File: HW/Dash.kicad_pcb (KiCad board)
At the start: 4 copper layers, 81 x 56 mm, 104 parts, among them J1 Conn_02x05_Top_Bottom, J2 souriau18pin, Q1 Q_NMOS_GSD, Q10 Q_NMOS_GSD, Q11 Q_NMOS_GSD, Q12 BC857BDW1, Q13 Q_PMOS_GSD, Q14 Q_NMOS_GSD, Q15 Q_NMOS_GSD, Q2 Q_NMOS_GSD, Q3 Q_NMOS_GSD, Q4 Q_NMOS_GSD, Q5 Q_NMOS_GSD, Q6 Q_NMOS_GSD, Q7 Q_NMOS_GSD, Q8 Q_NMOS_GSD, Q9 Q_NMOS_GSD, SW1 SW_Push_Dual, U1 STM32F303VCTx, U2 SN65HVD234, U3 LM1117-3.3, U4 24AA02-OT, U5 LMZ14202TZE-ADJ_NOPB

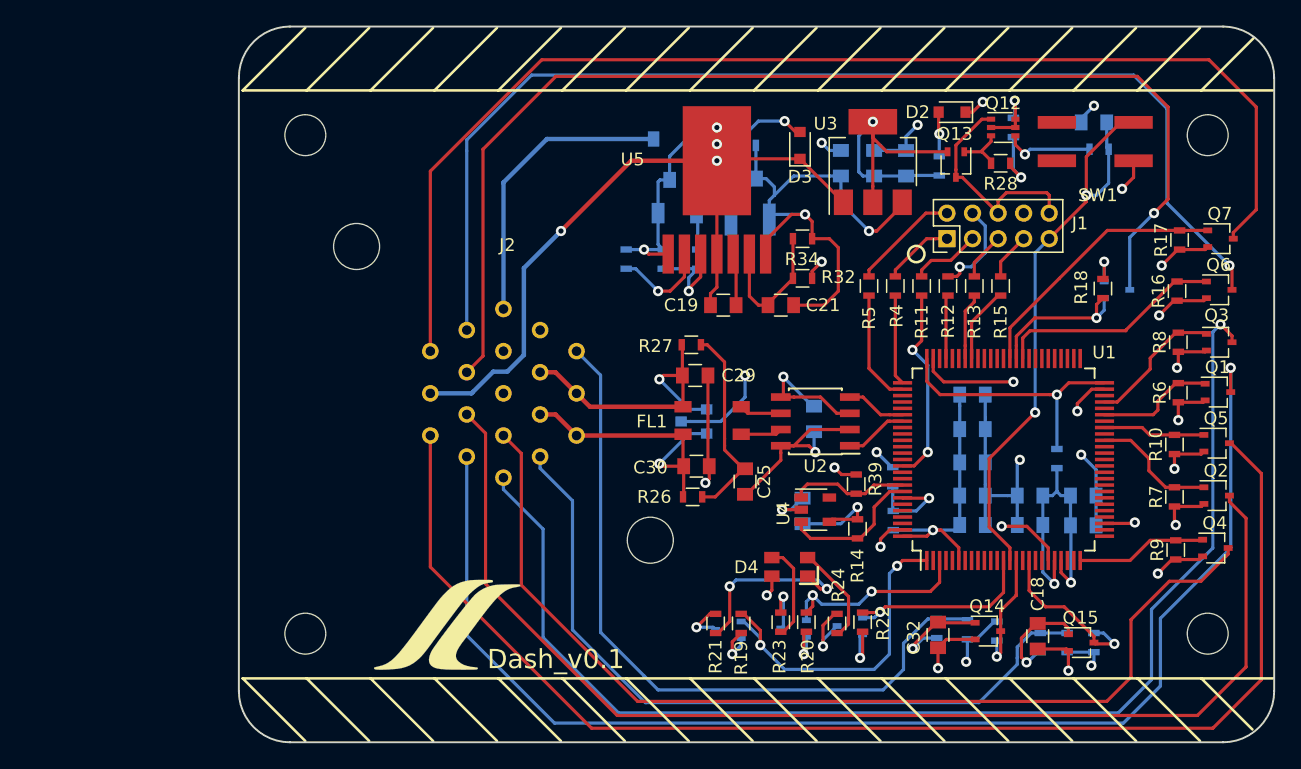
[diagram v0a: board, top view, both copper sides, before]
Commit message: Version 1.1
Version 1.1
Hw and Sw improvements
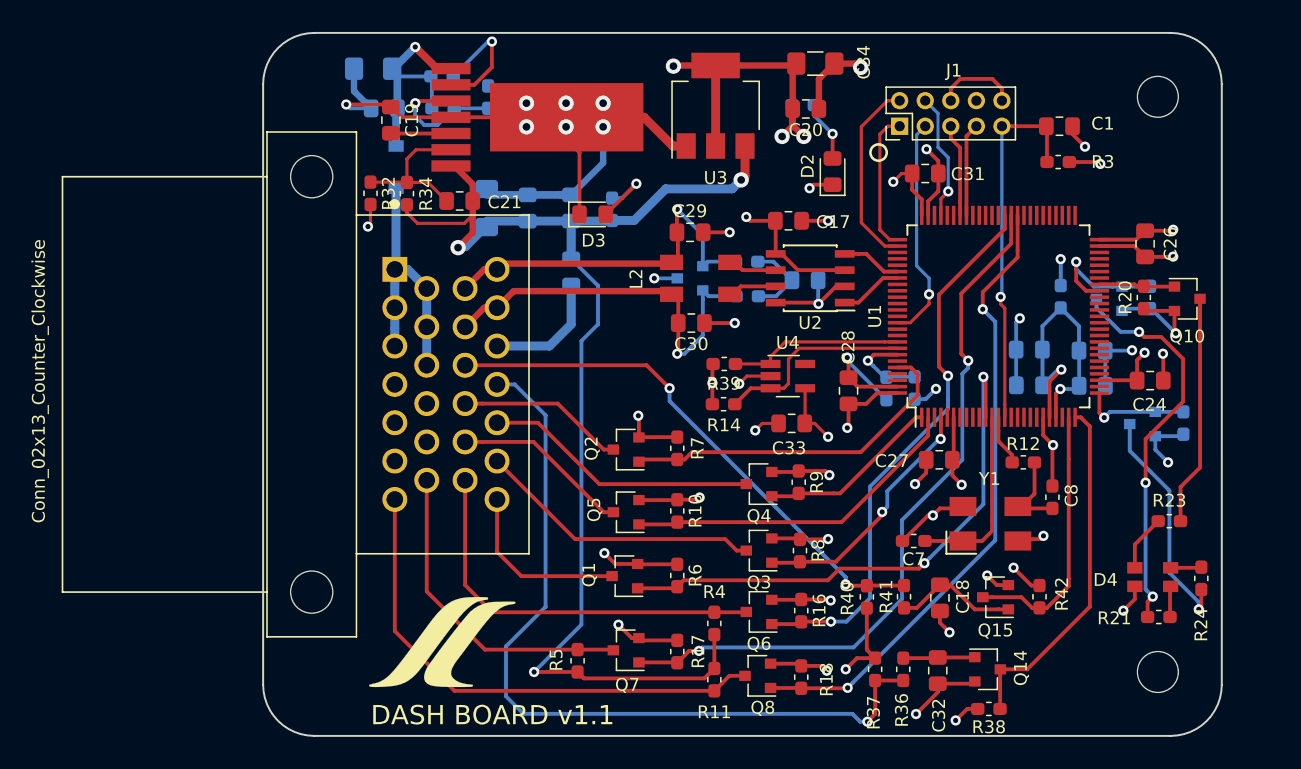
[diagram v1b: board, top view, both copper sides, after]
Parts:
- removed FL1: ACT45B-220-2P-TL003, footprint:ACT45B
- removed the G*** at (115.4, 97.7)
- removed the G*** at (123.6, 97.7)
- removed Q12: BC857BDW1, TO_SOT_Packages_SMD:SOT-363_SC-70-6
- removed Q13: Q_PMOS_GSD, TO_SOT_Packages_SMD:SOT-323_SC-70
- removed R13, R15: 22, Resistors_SMD:R_0603
- removed R25, R28: 68.1k, Resistors_SMD:R_0603
- removed the REF** at (174.9, 98.4)
- removed the REF** at (174.9, 59.4)
- removed the REF** at (104.3, 59.4)
- removed the REF** at (104.3, 98.4)
- removed SW1: SW_Push_Dual, footprint:pulsante
- added C7: 10p, Capacitor_SMD:C_0603_1608Metric_Pad1.05x0.95mm_HandSolder, F.Cu at (151.9, 91.2)
- added C8: 10p, Capacitor_SMD:C_0603_1608Metric_Pad1.05x0.95mm_HandSolder, F.Cu at (162.8, 87.7)
- added F1: Fuse, Fuse:Fuse_0805_2012Metric_Pad1.15x1.40mm_HandSolder, B.Cu at (125.1, 70.1)
- added G***: LOGO, footprint:LOGO_little, F.Cu at (115.0, 99.0)
- added L2: L_Core_Ferrite_Coupled, footprint:ACT45B, F.Cu at (137.5, 71.8)
- added REF**: MountingHole_3.2mm_M3, MountingHole:MountingHole_3.2mm_M3, F.Cu at (171.0, 56.4)
- added REF**: MountingHole_3.2mm_M3, MountingHole:MountingHole_3.2mm_M3, F.Cu at (171.0, 101.4)
- added Y1: Crystal_GND24, footprint:Crystal_SMD_Abracon_ABM3B-4Pin_5.0x3.2mm, F.Cu at (157.9, 89.8)
- C1, C17, C20, C24, C26, C27, C28, C31, C33: footprint Capacitors_SMD:C_0805 -> Capacitor_SMD:C_0805_2012Metric_Pad1.15x1.40mm_HandSolder; moved to F.Cu
- C15, C16, C18, C19, C2, C21, C22, C29, C3, C30, C32, C4, C5: footprint Capacitors_SMD:C_0805 -> Capacitor_SMD:C_0805_2012Metric_Pad1.15x1.40mm_HandSolder
- C23: footprint Capacitors_SMD:C_1210 -> Capacitor_SMD:C_1206_3216Metric_Pad1.42x1.75mm_HandSolder
- C25: footprint Capacitors_SMD:C_0805 -> Capacitor_SMD:C_0805_2012Metric_Pad1.15x1.40mm_HandSolder; moved to B.Cu
- C34: footprint Capacitors_SMD:C_0805 -> Capacitor_SMD:C_1206_3216Metric_Pad1.42x1.75mm_HandSolder; moved to F.Cu
- C6: footprint Capacitors_SMD:C_1206 -> Capacitor_SMD:C_1206_3216Metric_Pad1.42x1.75mm_HandSolder
- D1: footprint Diodes_SMD:D_SOD-123 -> Diode_SMD:D_SOD-123
- D2, D3: footprint Diodes_SMD:D_0805 -> LED_SMD:LED_0805_2012Metric_Pad1.15x1.40mm_HandSolder
- J2: value souriau18pin -> Conn_02x13_Counter_Clockwise; footprint footprint:8STA1418 -> 26pos:TE_9-6437287-8
- L1: footprint Inductors_SMD:L_0603 -> Inductor_SMD:L_0603_1608Metric_Pad1.05x0.95mm_HandSolder
- Q1, Q11, Q14, Q15, Q2, Q3, Q4, Q5, Q6, Q7, Q9: footprint TO_SOT_Packages_SMD:SOT-323_SC-70 -> Package_TO_SOT_SMD:SOT-23
- Q10, Q8: footprint TO_SOT_Packages_SMD:SOT-323_SC-70 -> Package_TO_SOT_SMD:SOT-23; moved to F.Cu
- R1, R10, R23, R24, R29, R30, R31, R32, R33, R34, R35, R6, R7, R8, R9: footprint Resistors_SMD:R_0603 -> Resistor_SMD:R_0603_1608Metric_Pad1.05x0.95mm_HandSolder
- R11, R4, R5: value 22 -> 3.3k; footprint Resistors_SMD:R_0603 -> Resistor_SMD:R_0603_1608Metric_Pad1.05x0.95mm_HandSolder
- R12: value 22 -> 0; footprint Resistors_SMD:R_0603 -> Resistor_SMD:R_0603_1608Metric_Pad1.05x0.95mm_HandSolder
- R14, R39: value 2k -> 3k; footprint Resistors_SMD:R_0603 -> Resistor_SMD:R_0603_1608Metric_Pad1.05x0.95mm_HandSolder
- R16, R17, R18, R20: value 100k -> 33k; footprint Resistors_SMD:R_0603 -> Resistor_SMD:R_0603_1608Metric_Pad1.05x0.95mm_HandSolder
- R19, R22: value 100k -> 33k; footprint Resistors_SMD:R_0603 -> Resistor_SMD:R_0603_1608Metric_Pad1.05x0.95mm_HandSolder; moved to B.Cu
- R2: value 15k -> 33k; footprint Resistors_SMD:R_0603 -> Resistor_SMD:R_0603_1608Metric_Pad1.05x0.95mm_HandSolder
- R21: value 1.6k -> 1.2k; footprint Resistors_SMD:R_0603 -> Resistor_SMD:R_0603_1608Metric_Pad1.05x0.95mm_HandSolder
- R26, R27: footprint Resistors_SMD:R_0603 -> Resistor_SMD:R_0603_1608Metric_Pad1.05x0.95mm_HandSolder; moved to B.Cu
- R3, R36, R37, R38, R40, R41, R42: footprint Resistors_SMD:R_0603 -> Resistor_SMD:R_0603_1608Metric_Pad1.05x0.95mm_HandSolder; moved to F.Cu
- U1: footprint Housings_QFP:LQFP-100_14x14mm_Pitch0.5mm -> Package_QFP:LQFP-100_14x14mm_P0.5mm
- U2: footprint Housings_SOIC:SOIC-8_3.9x4.9mm_Pitch1.27mm -> Package_SO:SOIC-8_3.9x4.9mm_P1.27mm
- U3: footprint TO_SOT_Packages_SMD:SOT-223 -> Package_TO_SOT_SMD:SOT-223
- U4: footprint TO_SOT_Packages_SMD:SOT-23-5 -> Package_TO_SOT_SMD:SOT-23-5_HandSoldering
- Z1: footprint TO_SOT_Packages_SMD:SOT-23 -> Package_TO_SOT_SMD:SOT-23
- moved Q7 56.6 mm to (129.4, 99.7), turned to 180 degrees
- moved R17 50.8 mm to (133.4, 99.8), turned to 270 degrees
- moved Q1 48.6 mm to (129.3, 93.9), turned to 180 degrees
- moved Q5 46.5 mm to (129.4, 88.9), turned to 180 degrees
- moved Q2 46.3 mm to (129.4, 84.0), turned to 180 degrees
- moved Q6 43.9 mm to (139.8, 96.7), turned to 180 degrees
- moved R6 41.7 mm to (133.4, 93.8), turned to 270 degrees
- moved Q8 41.3 mm to (139.7, 101.7), turned to 180 degrees
- moved R19 40.9 mm to (170.4, 72.1)
- moved Q10 40.2 mm to (173.3, 72.2), turned to 0 degrees
- moved Q3 39.5 mm to (139.8, 91.9), turned to 180 degrees
- moved Q9 39.5 mm to (167.2, 72.2)
- moved R10 39.2 mm to (133.4, 88.8), turned to 270 degrees
- moved R7 39.1 mm to (133.4, 83.9), turned to 270 degrees
- moved R16 38.6 mm to (143.1, 96.6), turned to 270 degrees
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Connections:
- C15 pad 1: /Power Supply/+5v -> +5V
- C21 pad 1: /Power Supply/+5v -> +5V
- C22 pad 1: /Power Supply/+5v -> +5V
- C23 pad 1: /Power Supply/+5v -> +5V
- C29 pad 1: /CAN_H -> /CAN_L
- C30 pad 2: /CAN_L -> /CAN_H
- J1 pad 1: Net-(J1-Pad1) -> /MCU/SWCLK
- J1 pad 10: /MCU/+3.3v_EXT -> +3V3
- J1 pad 2: Net-(J1-Pad2) -> /MCU/JTDI
- J1 pad 3: Net-(J1-Pad3) -> /MCU/SWO
- J1 pad 4: Net-(J1-Pad4) -> /MCU/SWDIO
- J1 pad 5: Net-(J1-Pad5) -> /MCU/USART_RX
- J1 pad 6: /MCU/+3.3v_EXT -> +3V3
- J1 pad 7: Net-(J1-Pad7) -> /MCU/USART_TX
- Q6 pad 1: /Cockpit management/PUMP_CMD -> /Cockpit management/PWM3
- Q6 pad 3: /PMP -> /PWM3
- Q7 pad 1: /Cockpit management/BP_FAN_CMD -> /Cockpit management/PWM2
- Q7 pad 3: /FAN -> /PWM2
- Q8 pad 1: /MCU/Fan_Rad_Cmd -> /Cockpit management/PWM1
- Q8 pad 3: /RAD -> /PWM1
- R11 pad 1: Net-(J1-Pad3) -> /PWM1
- R11 pad 2: /MCU/SWO -> +5V
- R12 pad 1: Net-(J1-Pad4) -> Net-(R12-Pad1)
- R12 pad 2: /MCU/SWDIO -> Net-(C8-Pad1)
- R16 pad 2: /Cockpit management/PUMP_CMD -> /Cockpit management/PWM3
- R17 pad 2: /Cockpit management/BP_FAN_CMD -> /Cockpit management/PWM2
- R18 pad 2: /MCU/Fan_Rad_Cmd -> /Cockpit management/PWM1
- R26 pad 1: /CAN_L -> /CAN_H
- R27 pad 1: /CAN_H -> /CAN_L
- R34 pad 2: /Power Supply/+5v -> +5V
- R35 pad 1: /Power Supply/+5v -> +5V
- R4 pad 1: Net-(J1-Pad1) -> /PWM3
- R4 pad 2: /MCU/SWCLK -> +5V
- R5 pad 1: Net-(J1-Pad2) -> /PWM2
- R5 pad 2: /MCU/JTDI -> +5V
- U1 pad 1: /MCU/gpio_RED -> /Cockpit management/BUZZER_CMD
- U1 pad 11: Net-(U1-Pad11) -> /Cockpit management/IMD_LED_CMD
- U1 pad 13: /MCU/gpio_BLUE -> Net-(R12-Pad1)
- U1 pad 15: /MCU/RTD_Button -> Net-(U1-Pad15)
- U1 pad 17: /Cockpit management/Spare_Button -> Net-(U1-Pad17)
- U1 pad 2: Net-(U1-Pad2) -> /Cockpit management/NO_HV_LED_CMD
- U1 pad 24: Net-(U1-Pad24) -> /Cockpit management/Spare_Button
- U1 pad 25: /Cockpit management/BUZZER_CMD -> /MCU/RTD_Button
- U1 pad 26: Net-(U1-Pad26) -> /MCU/gpio_BLUE
- U1 pad 3: /MCU/gpio_GREEN -> Net-(U1-Pad3)
- U1 pad 4: Net-(U1-Pad4) -> /Cockpit management/RTD_LED_CMD
- U1 pad 41: /Cockpit management/BMS_LED_CMD -> Net-(U1-Pad41)
- U1 pad 42: Net-(U1-Pad42) -> /MCU/gpio_RED
- U1 pad 43: /Cockpit management/NO_HV_LED_CMD -> /MCU/gpio_GREEN
- U1 pad 45: /Cockpit management/IMD_LED_CMD -> Net-(U1-Pad45)
- U1 pad 47: /Cockpit management/RTD_LED_CMD -> Net-(U1-Pad47)
- U1 pad 60: /Cockpit management/PUMP_CMD -> /Cockpit management/PWM1
- U1 pad 61: /MCU/Fan_Rad_Cmd -> /Cockpit management/PWM2
- U1 pad 62: /Cockpit management/BP_FAN_CMD -> /Cockpit management/PWM3
- U1 pad 96: Net-(U1-Pad96) -> /Cockpit management/BMS_LED_CMD
- U3 pad 3: /Power Supply/+5v -> +5V
- U5 pad 7: /Power Supply/+5v -> +5V
- Z1 pad 1: /CAN_H -> /CAN_L
- Z1 pad 2: /CAN_L -> /CAN_H
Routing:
- net +5V: track 0.00 -> 97.6 mm, vias 0 -> 3
- net /FAN: track 94.9 -> 0.00 mm
- net /RAD: track 90.5 -> 0.00 mm, vias 1 -> 0
- net /PMP: track 89.1 -> 0.00 mm, vias 1 -> 0
- net /HV_LED: track 101.7 -> 13.9 mm
- net /IMD_LED: track 101.4 -> 13.9 mm, vias 1 -> 0
- net /BMS_LED: track 93.1 -> 13.1 mm
- net /RTD_LED: track 96.7 -> 22.4 mm, vias 1 -> 0
- net /BUZ: track 79.2 -> 21.5 mm
- net /Cockpit management/PWM2: track 0.00 -> 56.7 mm, vias 0 -> 2
- net /Cockpit management/PWM1: track 0.00 -> 49.3 mm, vias 0 -> 2
- net /Cockpit management/PWM3: track 0.00 -> 43.4 mm, vias 0 -> 2
- net /Power Supply/+5v: track 41.3 -> 0.00 mm, vias 2 -> 0
- net /PWM1: track 0.00 -> 40.1 mm
- net /Cockpit management/IMD_LED_CMD: track 9.33 -> 43.0 mm, vias 0 -> 2
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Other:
- board size 81 x 56 mm -> 75 x 55 mm
- net class Default added: clearance 0.2, trace_width 0.3, via_dia 0.8, via_drill 0.4
- board text added: "DASH BOARD v1.1"
- board text removed: "Dash_v0.1"
